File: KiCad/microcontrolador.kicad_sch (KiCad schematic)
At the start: 17 parts, among them J2 DE9_Pins_MountingHoles, J3 Conn_01x05, J5 DE9_Pins_MountingHoles, U4 MCP2551-I-SN, U7 PIC24HJ128GP502, Y1 8MHz

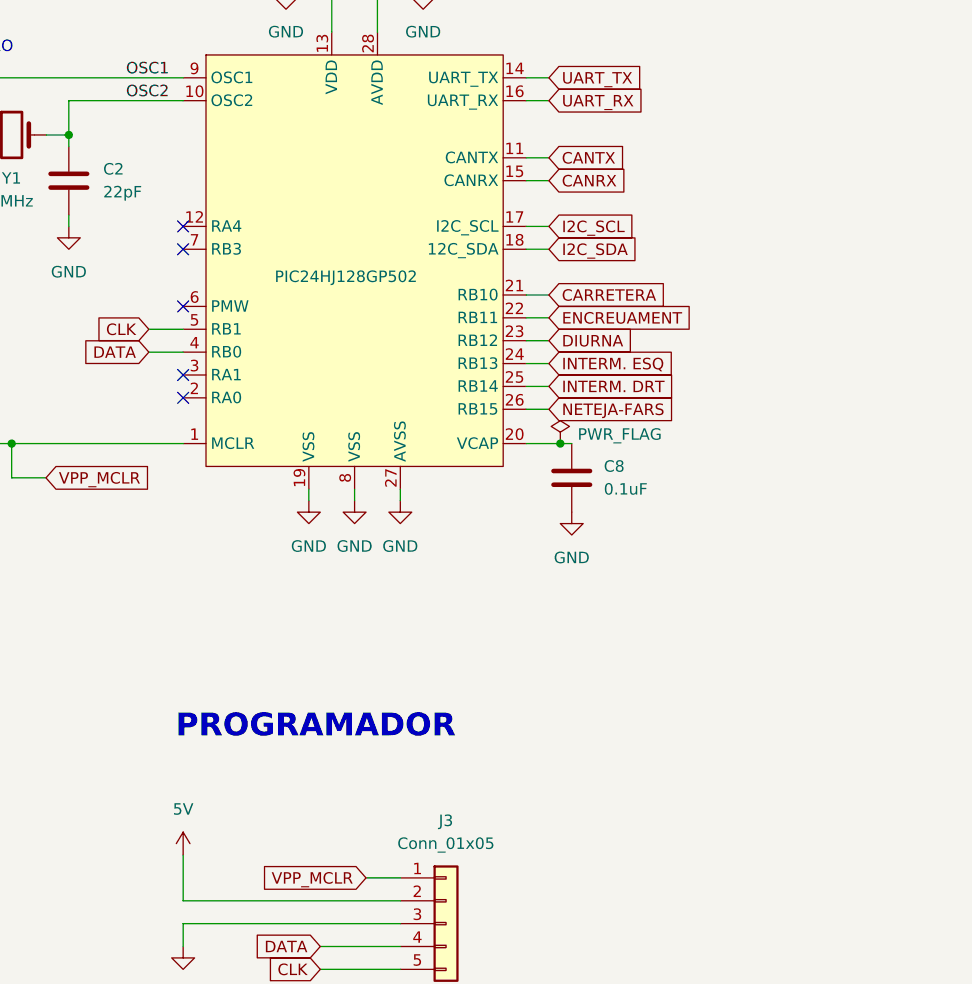
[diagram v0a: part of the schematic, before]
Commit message: algo de routing
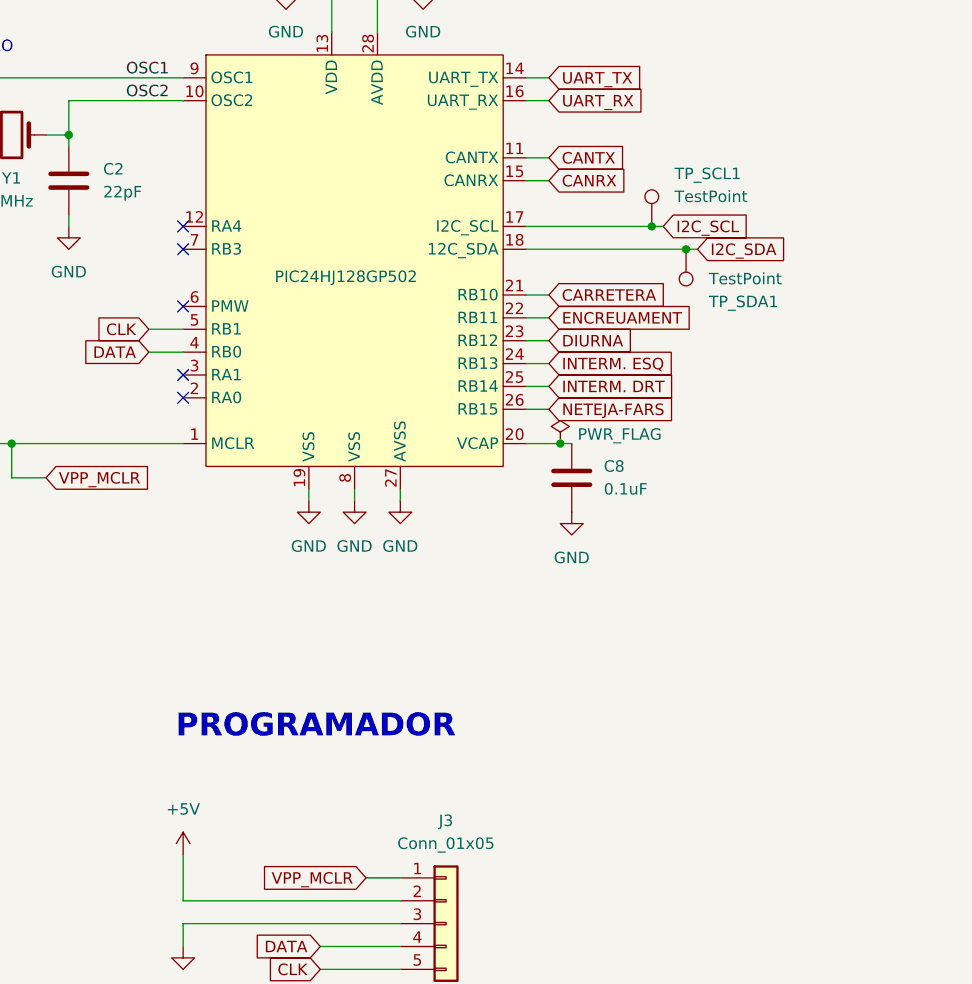
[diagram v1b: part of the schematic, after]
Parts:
- added TP_SCL1, TP_SDA1: TestPoint, Connector_PinHeader_2.54mm:PinHeader_1x01_P2.54mm_Vertical, symbol Connector:TestPoint
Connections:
- net 5V is gone; now on net +5V: J3.2 (Pin_2)
- net I2C_SCL: now also TP_SCL1.1
- net I2C_SDA: now also TP_SDA1.1
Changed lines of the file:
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@@
+	)
+	(junction
+		(at 142.24 90.17)
+		(diameter 0)
+		(color 0 0 0 0)
 	)
 	(junction
@@
 		(color 0 0 0 0)
 	)
+	(junction
+		(at 146.05 92.71)
+		(diameter 0)
+		(color 0 0 0 0)
+	)
 	(no_connect
 		(at 236.22 113.03)
@@
 	(wire
 		(pts
+			(xy 146.05 92.71) (xy 147.32 92.71)
+		)
+		(stroke
+			(width 0)
+			(type default)
+		)
+	)
+	(wire
+		(pts
 			(xy 232.41 110.49) (xy 232.41 111.76)
 		)
@@
 	(wire
 		(pts
+			(xy 128.27 92.71) (xy 146.05 92.71)
+		)
+		(stroke
+			(width 0)
+			(type default)
+		)
+	)
+	(wire
+		(pts
 			(xy 215.9 128.27) (xy 219.71 128.27)
 		)
@@
 	(wire
 		(pts
-			(xy 130.81 92.71) (xy 128.27 92.71)
-		)
-		(stroke
-			(width 0)
-			(type default)
-		)
-	)
-	(wire
-		(pts
 			(xy 130.81 85.09) (xy 128.27 85.09)
 		)
@@
 	(wire
 		(pts
+			(xy 128.27 90.17) (xy 142.24 90.17)
+		)
+		(stroke
+			(width 0)
+			(type default)
+		)
+	)
+	(wire
+		(pts
 			(xy 71.12 118.11) (xy 71.12 114.3)
 		)
@@
 	(wire
 		(pts
-			(xy 130.81 90.17) (xy 128.27 90.17)
+			(xy 143.51 90.17) (xy 142.24 90.17)
 		)
 		(stroke
@@
 	(global_label "I2C_SDA"
 		(shape input)
-		(at 130.81 92.71 0)
+		(at 147.32 92.71 0)
 		(fields_autoplaced yes)
 		(effects
@@
 		)
 		(property "Intersheetrefs" "${INTERSHEET_REFS}"
-			(at 141.4152 92.71 0)
+			(at 157.9252 92.71 0)
 			(effects
 				(font
@@
 	(global_label "I2C_SCL"
 		(shape input)
-		(at 130.81 90.17 0)
+		(at 143.51 90.17 0)
 		(fields_autoplaced yes)
 		(effects
@@
 		)
 		(property "Intersheetrefs" "${INTERSHEET_REFS}"
-			(at 141.3547 90.17 0)
+			(at 154.0547 90.17 0)
 			(effects
 				(font
@@
 	)
 	(symbol
+		(lib_id "Connector:TestPoint")
+		(at 142.24 90.17 0)
+		(unit 1)
+		(exclude_from_sim no)
+		(in_bom yes)
+		(on_board yes)
+		(dnp no)
+		(property "Reference" "TP_SCL1"
+			(at 144.78 84.328 0)
+			(effects
+				(font
+					(size 1.27 1.27)
+				)
+				(justify left)
+			)
+		)
+		(property "Value" "TestPoint"
+			(at 144.78 86.868 0)
+			(effects
+				(font
+					(size 1.27 1.27)
+				)
+				(justify left)
+			)
+		)
+		(property "Footprint" "Connector_PinHeader_2.54mm:PinHeader_1x01_P2.54mm_Vertical"
+			(at 147.32 90.17 0)
+			(effects
+				(font
+					(size 1.27 1.27)
+				)
+				(hide yes)
+			)
+		)
+		(property "Datasheet" "~"
+			(at 147.32 90.17 0)
+			(effects
+				(font
+					(size 1.27 1.27)
+				)
+				(hide yes)
+			)
+		)
+		(property "Description" "test point"
+			(at 142.24 90.17 0)
+			(effects
+				(font
+					(size 1.27 1.27)
+				)
+				(hide yes)
+			)
+		)
+		(pin "1"
+		)
+		(instances
+			(project ""
+				(path "/b4874c87-978f-427f-bc45-3635f8629977/65403977-6a27-47ce-ace7-4876548c1d8f"
+					(reference "TP_SCL1")
+					(unit 1)
+				)
+			)
+		)
+	)
+	(symbol
 		(lib_id "Device:R")
 		(at 55.88 106.68 180)
@@
 				(path "/b4874c87-978f-427f-bc45-3635f8629977/65403977-6a27-47ce-ace7-4876548c1d8f"
 					(reference "R1")
+					(unit 1)
+				)
+			)
+		)
+	)
+	(symbol
+		(lib_id "Connector:TestPoint")
+		(at 146.05 92.71 0)
+		(mirror x)
+		(unit 1)
+		(exclude_from_sim no)
+		(in_bom yes)
+		(on_board yes)
+		(dnp no)
+		(property "Reference" "TP_SDA1"
+			(at 148.59 98.552 0)
+			(effects
+				(font
+					(size 1.27 1.27)
+				)
+				(justify left)
+			)
+		)
+		(property "Value" "TestPoint"
+			(at 148.59 96.012 0)
+			(effects
+				(font
+					(size 1.27 1.27)
+				)
+				(justify left)
+			)
+		)
+		(property "Footprint" "Connector_PinHeader_2.54mm:PinHeader_1x01_P2.54mm_Vertical"
+			(at 151.13 92.71 0)
+			(effects
+				(font
+					(size 1.27 1.27)
+				)
+				(hide yes)
+			)
+		)
+		(property "Datasheet" "~"
+			(at 151.13 92.71 0)
+			(effects
+				(font
+					(size 1.27 1.27)
+				)
+				(hide yes)
+			)
+		)
+		(property "Description" "test point"
+			(at 146.05 92.71 0)
+			(effects
+				(font
+					(size 1.27 1.27)
+				)
+				(hide yes)
+			)
+		)
+		(pin "1"
+		)
+		(instances
+			(project "PROJECTE_LLUMS"
+				(path "/b4874c87-978f-427f-bc45-3635f8629977/65403977-6a27-47ce-ace7-4876548c1d8f"
+					(reference "TP_SDA1")
 					(unit 1)
 				)
@@
 			)
 		)
-		(property "Value" "5V"
+		(property "Value" "+5V"
 			(at 90.17 154.94 0)
 			(effects
